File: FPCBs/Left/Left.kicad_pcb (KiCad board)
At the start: 2 copper layers, 46.9 x 13.4 mm, 7 parts, among them J1 To PCB, SW1 SW_Rotary_1x6_MP

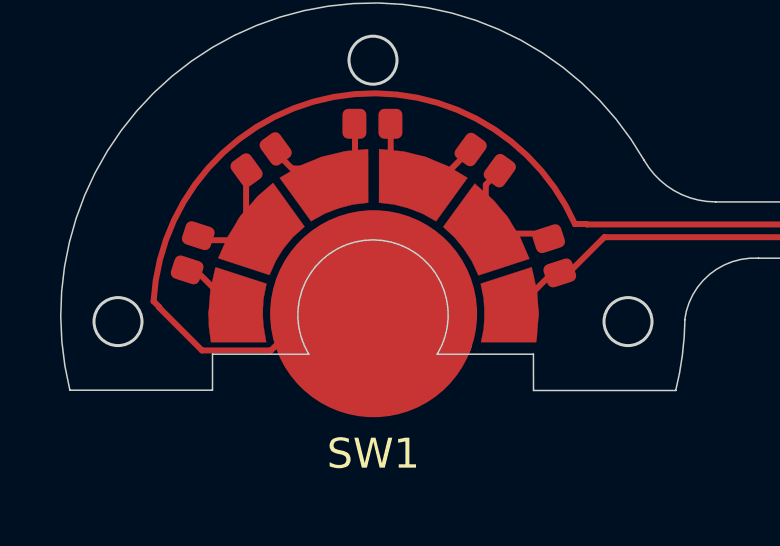
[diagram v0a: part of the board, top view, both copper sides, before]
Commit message: Add copper tot he back side
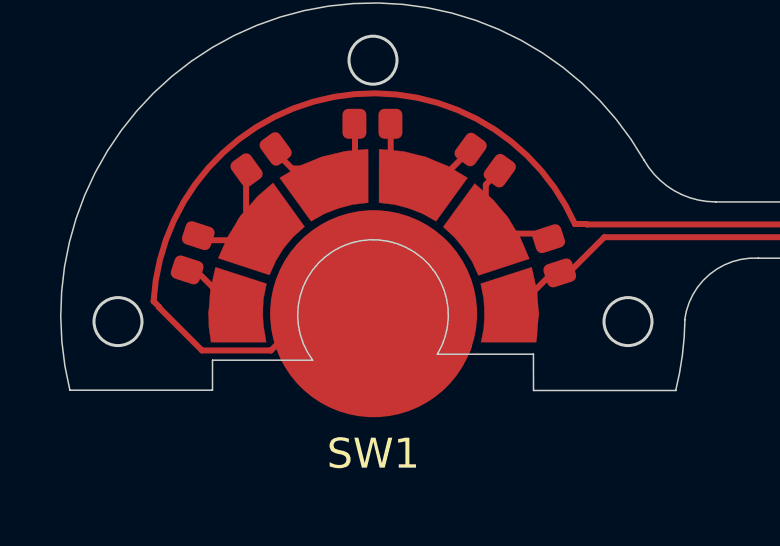
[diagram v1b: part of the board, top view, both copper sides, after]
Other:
- outline, holes or cut-outs redrawn
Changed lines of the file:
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@@
 		(tenting front back)
 		(pcbplotparams
-			(layerselection 0x00000000_00000000_55f55555_5755f5ff)
+			(layerselection 0x00000000_00000000_55555555_5755f5ff)
 			(plot_on_all_layers_selection 0x00000000_00000000_00000000_00000000)
 			(disableapertmacros no)
@@
 			(usegerberattributes yes)
 			(usegerberadvancedattributes yes)
-			(creategerberjobfile yes)
+			(creategerberjobfile no)
 			(dashed_line_dash_ratio 12.000000)
 			(dashed_line_gap_ratio 3.000000)
@@
 			(sketchdnponfab yes)
 			(crossoutdnponfab yes)
-			(subtractmaskfromsilk no)
+			(subtractmaskfromsilk yes)
 			(outputformat 1)
 			(mirror no)
 			(drillshape 0)
 			(scaleselection 1)
-			(outputdirectory "export/drills/")
+			(outputdirectory "Gerber/")
 		)
 	)
@@
 	)
 	(gr_arc
-		(start 106.36 101.3)
-		(mid 108.5 97.488487)
-		(end 110.64 101.3)
+		(start 106.49 101.5)
+		(mid 108.380646 97.486841)
+		(end 110.643829 101.302335)
 		(stroke
 			(width 0.05)
@@
 	)
 	(gr_line
-		(start 103.15 101.3)
+		(start 103.15 101.5)
 		(end 103.15 102.5)
 		(stroke
@@
 	)
 	(gr_line
-		(start 106.36 101.3)
-		(end 103.15 101.3)
+		(start 106.49 101.5)
+		(end 103.15 101.5)
 		(stroke
 			(width 0.05)
-			(type default)
+			(type solid)
 		)
 		(layer "Edge.Cuts")
